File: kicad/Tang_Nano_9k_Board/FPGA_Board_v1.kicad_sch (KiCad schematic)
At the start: 18 parts, among them J1 Conn_01x24, J2 Conn_01x24, J3 Conn_01x08, J4 Conn_01x04, J5 Conn_01x04, J6 Conn_01x04, J7 Conn_01x04, SW1 SW_DIP_x08, SW2 SW_Push, SW3 SW_Push, SW4 SW_Push

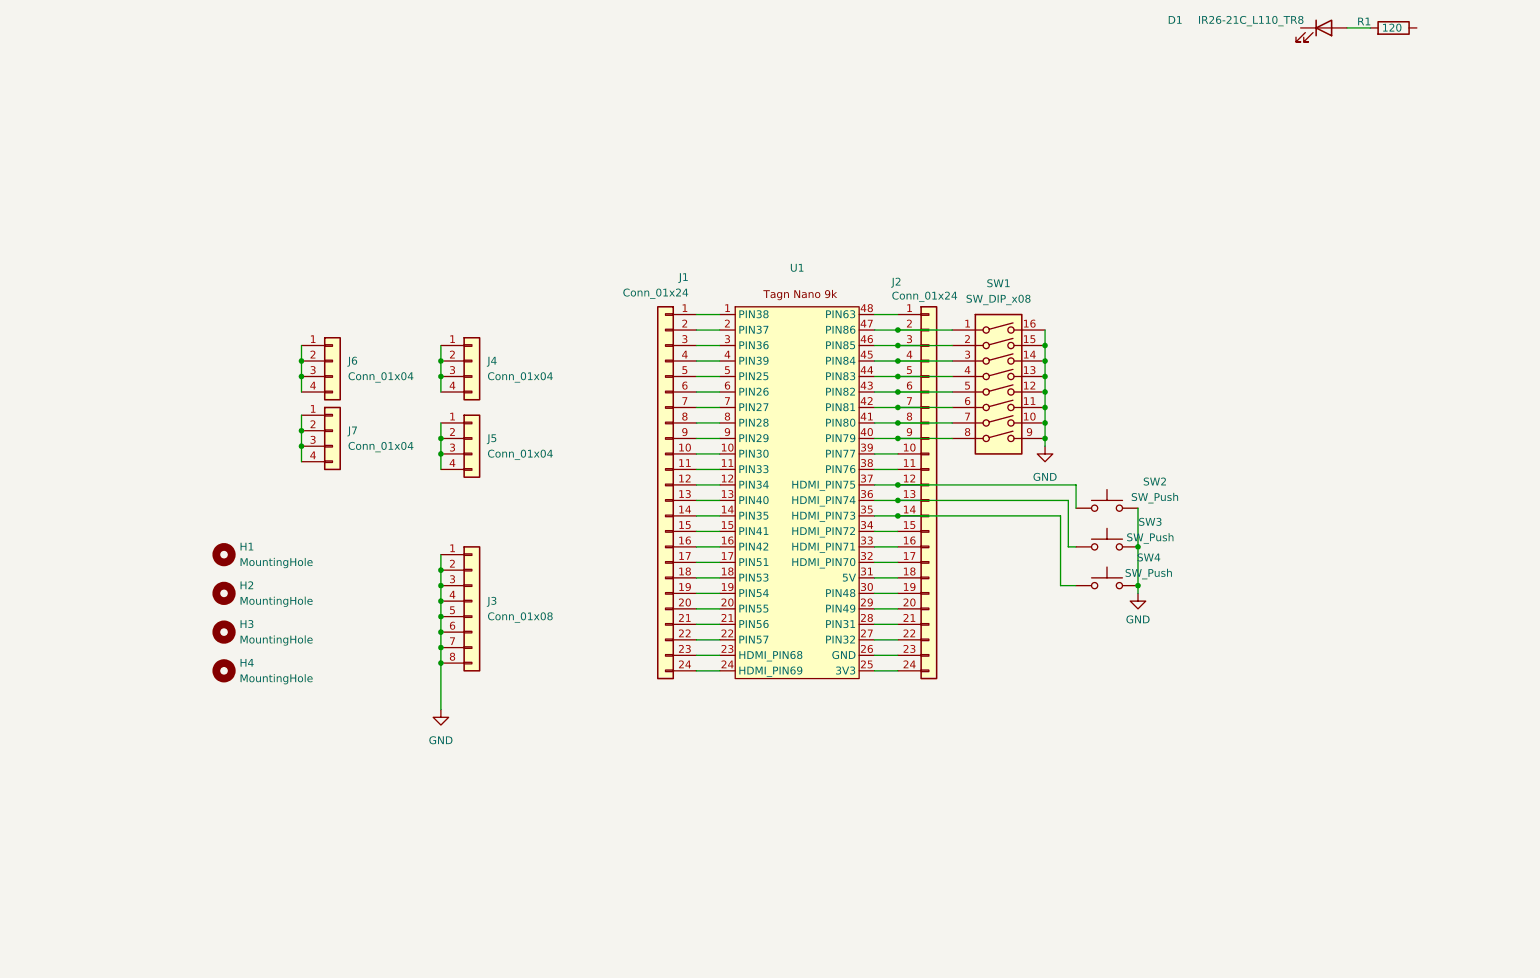
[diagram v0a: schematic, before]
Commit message: add led
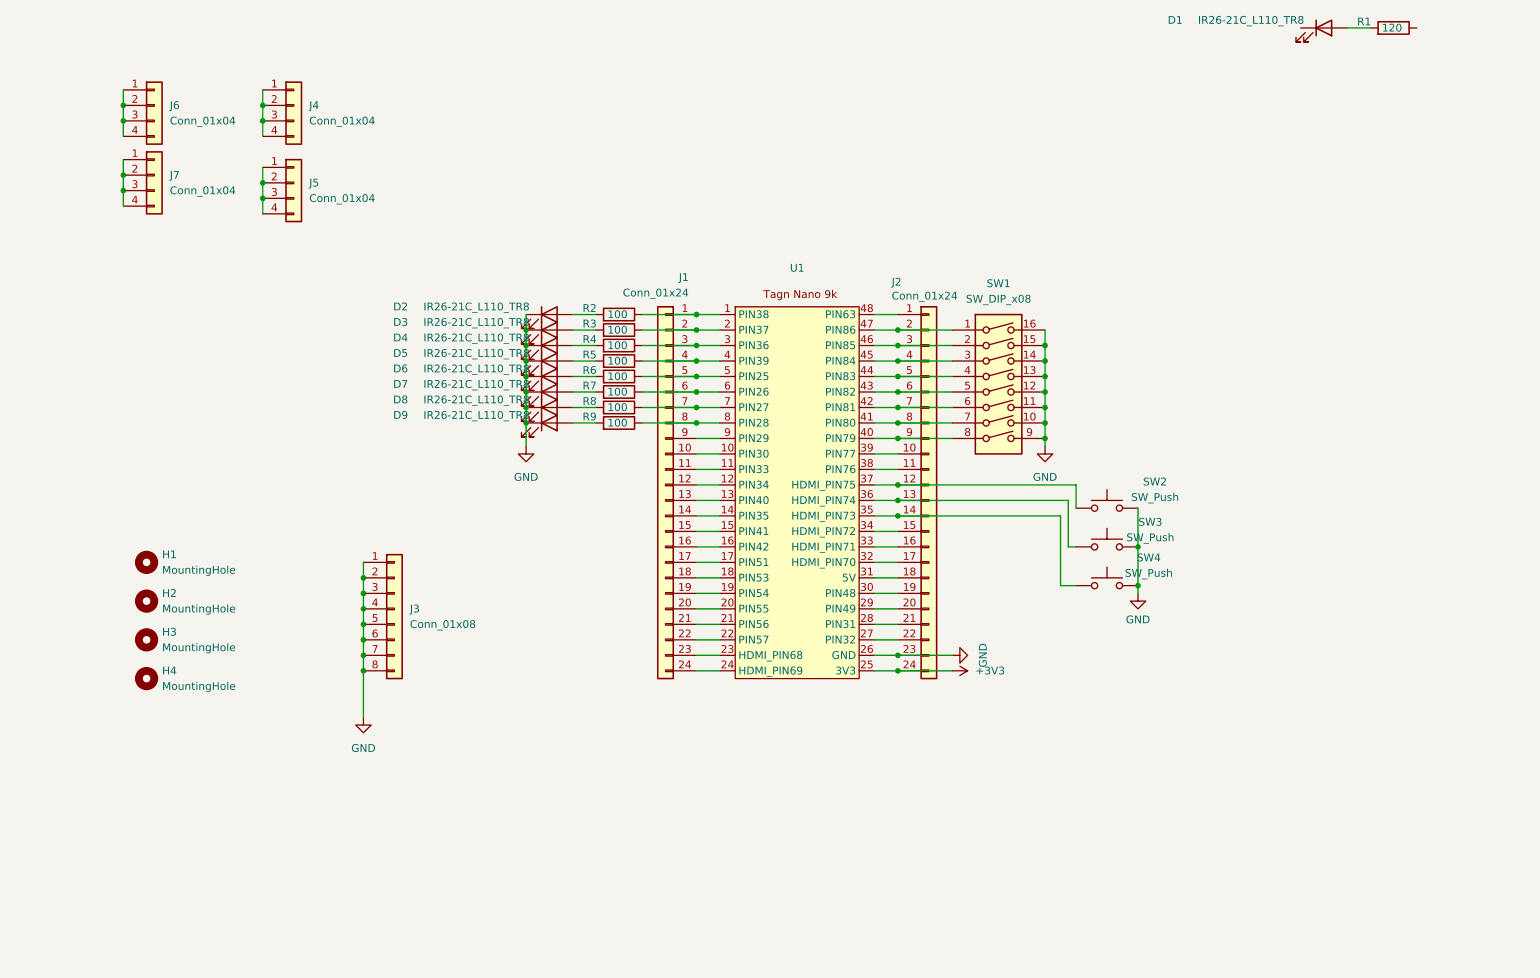
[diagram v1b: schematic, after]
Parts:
- added D2, D3, D4, D5, D6, D7, D8, D9: IR26-21C_L110_TR8, LED_SMD:LED_1206_3216Metric, symbol LED:IR26-21C_L110_TR8
- added R2, R3, R4, R5, R6, R7, R8, R9: 100, symbol Device:R
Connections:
- net GND: now also J2.23 (Pin_23), U1.26 (GND), D2.1 (K), D3.1 (K), D4.1 (K), D5.1 (K), D6.1 (K), D7.1 (K), D8.1 (K), D9.1 (K)
- net at J1.1 (Pin_1), U1.1 (PIN38): now also R2.1
- net at J1.2 (Pin_2), U1.2 (PIN37): now also R3.1
- net at J1.3 (Pin_3), U1.3 (PIN36): now also R4.1
- net at J1.4 (Pin_4), U1.4 (PIN39): now also R5.1
- net at J1.5 (Pin_5), U1.5 (PIN25): now also R6.1
- net at J1.6 (Pin_6), U1.6 (PIN26): now also R7.1
- net at J1.7 (Pin_7), U1.7 (PIN27): now also R8.1
- net at J1.8 (Pin_8), U1.8 (PIN28): now also R9.1
- net +3V3: now reaches J2.24 (Pin_24), U1.25 (3V3)
- new net: D6.2 (A), R6.2
- new net: D7.2 (A), R7.2
- new net: D8.2 (A), R8.2
- new net: D3.2 (A), R3.2
- new net: D4.2 (A), R4.2
- new net: D9.2 (A), R9.2
- new net: D5.2 (A), R5.2
- new net: D2.2 (A), R2.2
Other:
- moved on the sheet: H1, H2, H3, H4, J3, J4, J5, J6, J7

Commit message: update
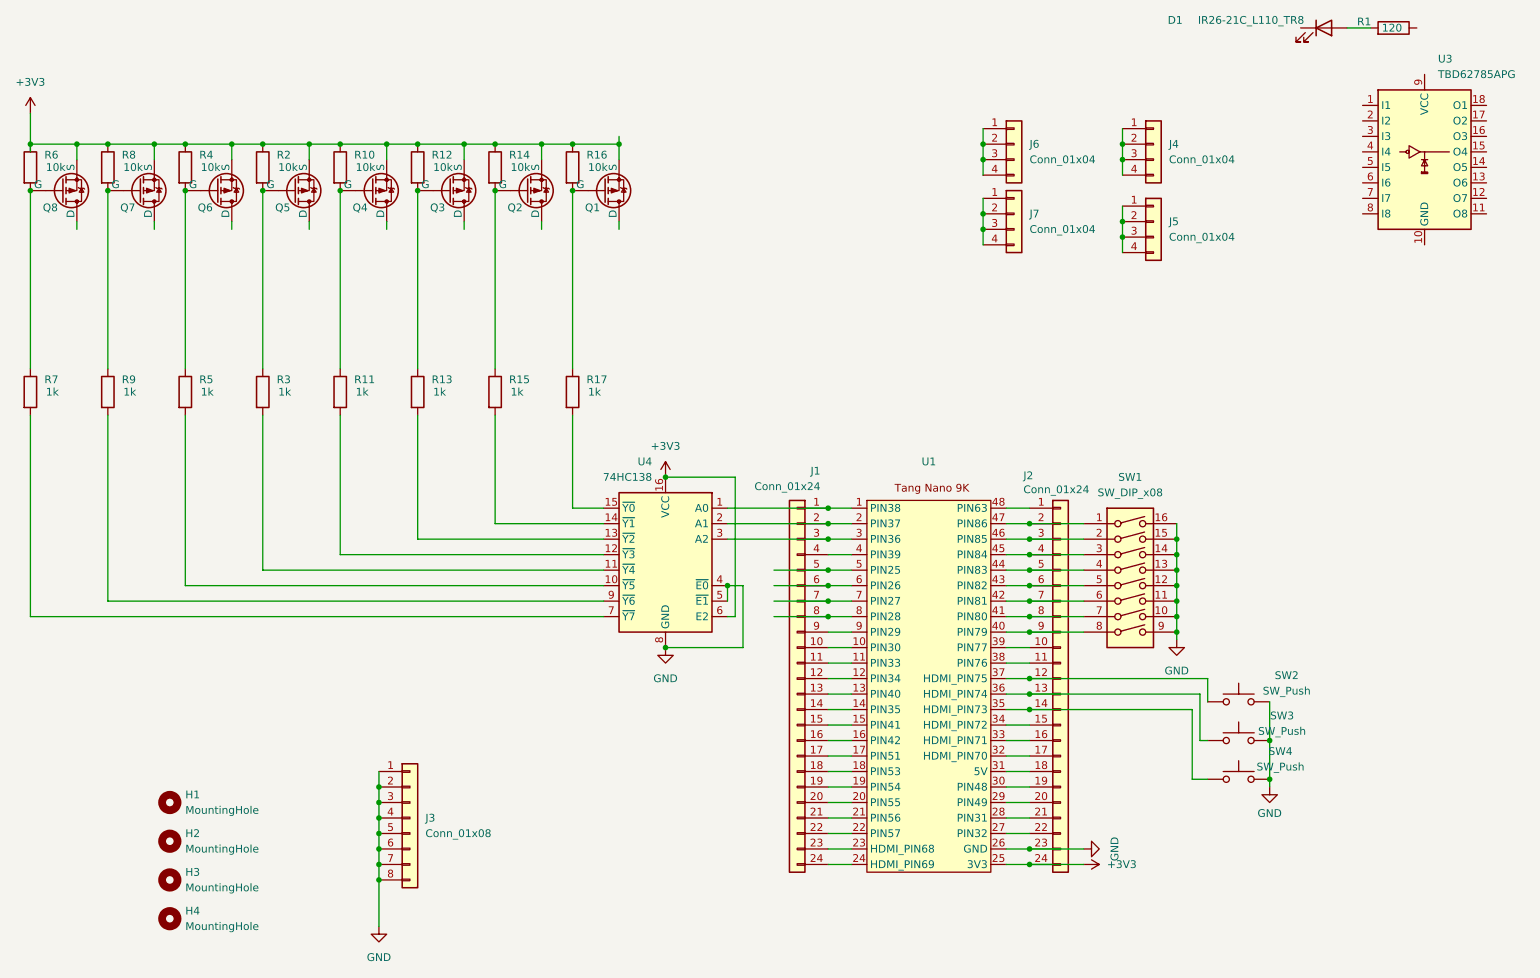
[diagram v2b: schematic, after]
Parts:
- removed D2, D3, D4, D5, D6, D7, D8, D9: IR26-21C_L110_TR8, LED_SMD:LED_1206_3216Metric, symbol LED:IR26-21C_L110_TR8
- removed U1: ~, symbol yuma_bf:Tang_Nano_9k
- added Q1, Q2, Q3, Q4, Q5, Q6, Q7, Q8: PMOS, symbol Simulation_SPICE:PMOS
- added R10, R12, R14, R16: 10k, symbol Device:R
- added R11, R13, R15, R17: 1k, symbol Device:R
- added U1: ~, symbol yuma_bf:Tang_Nano_9K
- added U3: TBD62785APG, Package_DIP:DIP-18_W7.62mm, symbol Transistor_Array:TBD62785APG
- added U4: 74HC138, symbol 74xx:74HC138
- R2, R4, R6, R8: value 100 -> 10k
- R3, R5, R7, R9: value 100 -> 1k
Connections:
- net +3V3: now also R2.1, R4.1, R6.1, R8.1, Q1.3 (S), Q2.3 (S), Q3.3 (S), Q4.3 (S), Q5.3 (S), Q6.3 (S), Q7.3 (S), Q8.3 (S), R10.1, R12.1, R14.1, R16.1, U1.25 (3V3), U4.16 (VCC), U4.6 (E2)
- net GND: now also U1.26 (GND), U4.4 (~{E0}), U4.5 (~{E1}), U4.8 (GND)
- net at R6.2: now also R7.1, Q8.2 (G)
- net at R7.2: now also U4.7 (~{Y7})
- net at R8.2: now also R9.1, Q7.2 (G)
- net at J1.2 (Pin_2): now also U1.2 (PIN37), U4.2 (A1); no longer R3.1
- net at R3.2: now also U4.11 (~{Y4})
- net at J1.1 (Pin_1): now also U1.1 (PIN38), U4.1 (A0); no longer R2.1
- net at J1.10 (Pin_10): now also U1.10 (PIN30)
- net at J1.11 (Pin_11): now also U1.11 (PIN33)
- net at J1.12 (Pin_12): now also U1.12 (PIN34)
- net at J1.13 (Pin_13): now also U1.13 (PIN40)
- net at J1.14 (Pin_14): now also U1.14 (PIN35)
- net at J1.15 (Pin_15): now also U1.15 (PIN41)
- net at J1.16 (Pin_16): now also U1.16 (PIN42)
- net at J1.17 (Pin_17): now also U1.17 (PIN51)
- net at J1.18 (Pin_18): now also U1.18 (PIN53)
- net at J1.19 (Pin_19): now also U1.19 (PIN54)
- net at J1.20 (Pin_20): now also U1.20 (PIN55)
- net at J1.21 (Pin_21): now also U1.21 (PIN56)
- net at J1.22 (Pin_22): now also U1.22 (PIN57)
- net at J1.23 (Pin_23): now also U1.23 (HDMI_PIN68)
- net at J1.24 (Pin_24): now also U1.24 (HDMI_PIN69)
- net at J1.3 (Pin_3): now also U1.3 (PIN36), U4.3 (A2); no longer R4.1
- net at J1.4 (Pin_4): now also U1.4 (PIN39); no longer R5.1
- net at J1.5 (Pin_5): now also U1.5 (PIN25); no longer R6.1
- net at J1.6 (Pin_6): now also U1.6 (PIN26); no longer R7.1
- net at J1.7 (Pin_7): now also U1.7 (PIN27); no longer R8.1
- net at J1.8 (Pin_8): now also U1.8 (PIN28); no longer R9.1
- net at J1.9 (Pin_9): now also U1.9 (PIN29)
- net at R4.2: now also R5.1, Q6.2 (G)
- net at J2.2 (Pin_2), SW1.1: now also U1.47 (PIN86)
- net at J2.3 (Pin_3), SW1.2: now also U1.46 (PIN85)
- net at J2.4 (Pin_4), SW1.3: now also U1.45 (PIN84)
- net at J2.5 (Pin_5), SW1.4: now also U1.44 (PIN83)
- net at J2.6 (Pin_6), SW1.5: now also U1.43 (PIN82)
- net at J2.7 (Pin_7), SW1.6: now also U1.42 (PIN81)
- net at J2.8 (Pin_8), SW1.7: now also U1.41 (PIN80)
- net at J2.9 (Pin_9), SW1.8: now also U1.40 (PIN79)
- net at R9.2: now also U4.9 (~{Y6})
- net at J2.22 (Pin_22): now also U1.27 (PIN32)
- net at J2.21 (Pin_21): now also U1.28 (PIN31)
- net at J2.20 (Pin_20): now also U1.29 (PIN49)
- net at J2.19 (Pin_19): now also U1.30 (PIN48)
- net at J2.18 (Pin_18): now also U1.31 (5V)
- net at J2.17 (Pin_17): now also U1.32 (HDMI_PIN70)
- net at J2.16 (Pin_16): now also U1.33 (HDMI_PIN71)
- net at J2.15 (Pin_15): now also U1.34 (HDMI_PIN72)
- net at J2.14 (Pin_14), SW4.1: now also U1.35 (HDMI_PIN73)
- net at J2.13 (Pin_13), SW3.1: now also U1.36 (HDMI_PIN74)
- net at J2.12 (Pin_12), SW2.1: now also U1.37 (HDMI_PIN75)
- net at J2.11 (Pin_11): now also U1.38 (PIN76)
- net at J2.10 (Pin_10): now also U1.39 (PIN77)
- net at J2.1 (Pin_1): now also U1.48 (PIN63)
- net at R5.2: now also U4.10 (~{Y5})
- net at R2.2: now also R3.1, Q5.2 (G)
- new net: Q3.2 (G), R12.2, R13.1
- new net: R13.2, U4.13 (~{Y2})
- new net: Q1.2 (G), R16.2, R17.1
- new net: Q2.2 (G), R14.2, R15.1
- new net: R15.2, U4.14 (~{Y1})
- new net: Q4.2 (G), R10.2, R11.1
- new net: R11.2, U4.12 (~{Y3})
- new net: R17.2, U4.15 (~{Y0})
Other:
- moved on the sheet: H1, H2, H3, H4, J1, J2, J3, J4, J5, J6, J7, SW1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

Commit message: complete FPGA Board tmp
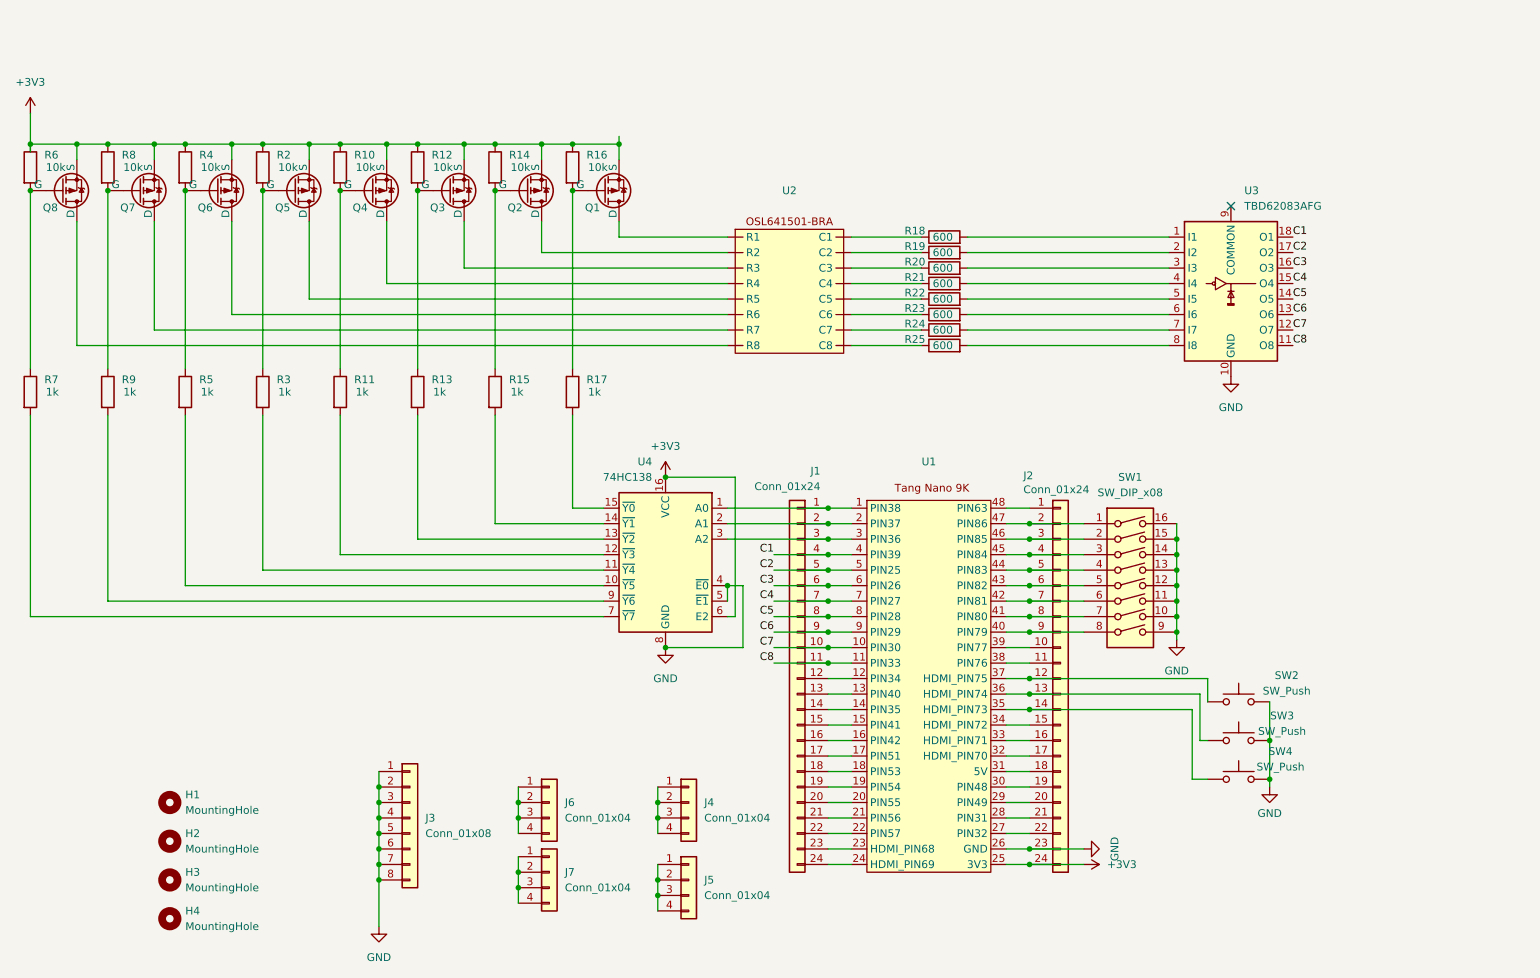
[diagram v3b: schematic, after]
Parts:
- removed D1: IR26-21C_L110_TR8, LED_SMD:LED_1206_3216Metric, symbol LED:IR26-21C_L110_TR8
- removed R1: 120, symbol Device:R
- removed U3: TBD62785APG, Package_DIP:DIP-18_W7.62mm, symbol Transistor_Array:TBD62785APG
- added R18, R19, R20, R21, R22, R23, R24, R25: 600, symbol Device:R
- added U2: ~, symbol yuma_bf:OSL641501-BRA
- added U3: TBD62083AFG, Package_DIP:DIP-18_W7.62mm, symbol yuma_bf:TBD62083AFG
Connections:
- net GND: now also U3.10 (GND)
- net at Q3.1 (D): now also U2. (R8)
- net C7: now reaches J1.10 (Pin_10), U1.10 (PIN30)
- net C7: now also U3.12 (O7)
- net C8: now reaches J1.11 (Pin_11), U1.11 (PIN33)
- net C8: now also U3.11 (O8)
- net C1: now reaches J1.4 (Pin_4), U1.4 (PIN39)
- net C1: now also U3.18 (O1)
- net C2: now reaches J1.5 (Pin_5), U1.5 (PIN25)
- net C2: now also U3.17 (O2)
- net C3: now reaches J1.6 (Pin_6), U1.6 (PIN26)
- net C3: now also U3.16 (O3)
- net C4: now reaches J1.7 (Pin_7), U1.7 (PIN27)
- net C4: now also U3.15 (O4)
- net C5: now reaches J1.8 (Pin_8), U1.8 (PIN28)
- net C5: now also U3.14 (O5)
- net C6: now reaches J1.9 (Pin_9), U1.9 (PIN29)
- net C6: now also U3.13 (O6)
- net at Q1.1 (D): now also U2. (R8)
- net at Q6.1 (D): now also U2. (R8)
- net at Q4.1 (D): now also U2. (R8)
- net at Q7.1 (D): now also U2. (R8)
- net at Q8.1 (D): now also U2. (R8)
- net at Q5.1 (D): now also U2. (R8)
- net at Q2.1 (D): now also U2. (R8)
- new net: R19.1, U2. (R8)
- new net: R25.1, U2. (R8)
- new net: R18.1, U2. (R8)
- new net: R24.1, U2. (R8)
- new net: R21.1, U2. (R8)
- new net: R20.1, U2. (R8)
- new net: R23.1, U2. (R8)
- new net: R22.1, U2. (R8)
- new net: R19.2, U3.2 (I2)
- new net: R25.2, U3.8 (I8)
- new net: R18.2, U3.1 (I1)
- new net: R20.2, U3.3 (I3)
- new net: R21.2, U3.4 (I4)
- new net: R22.2, U3.5 (I5)
- new net: R23.2, U3.6 (I6)
- new net: R24.2, U3.7 (I7)
- no-connect marks 0 -> 1
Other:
- moved on the sheet: J4, J5, J6, J7
